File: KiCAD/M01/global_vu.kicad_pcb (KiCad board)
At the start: 2 copper layers, 100 x 49 mm, 70 parts, among them J1 Conn_01x05, J2 Conn_01x05, U1 74HC595, U2 74HC595, U3 74HC595, U4 74HC595

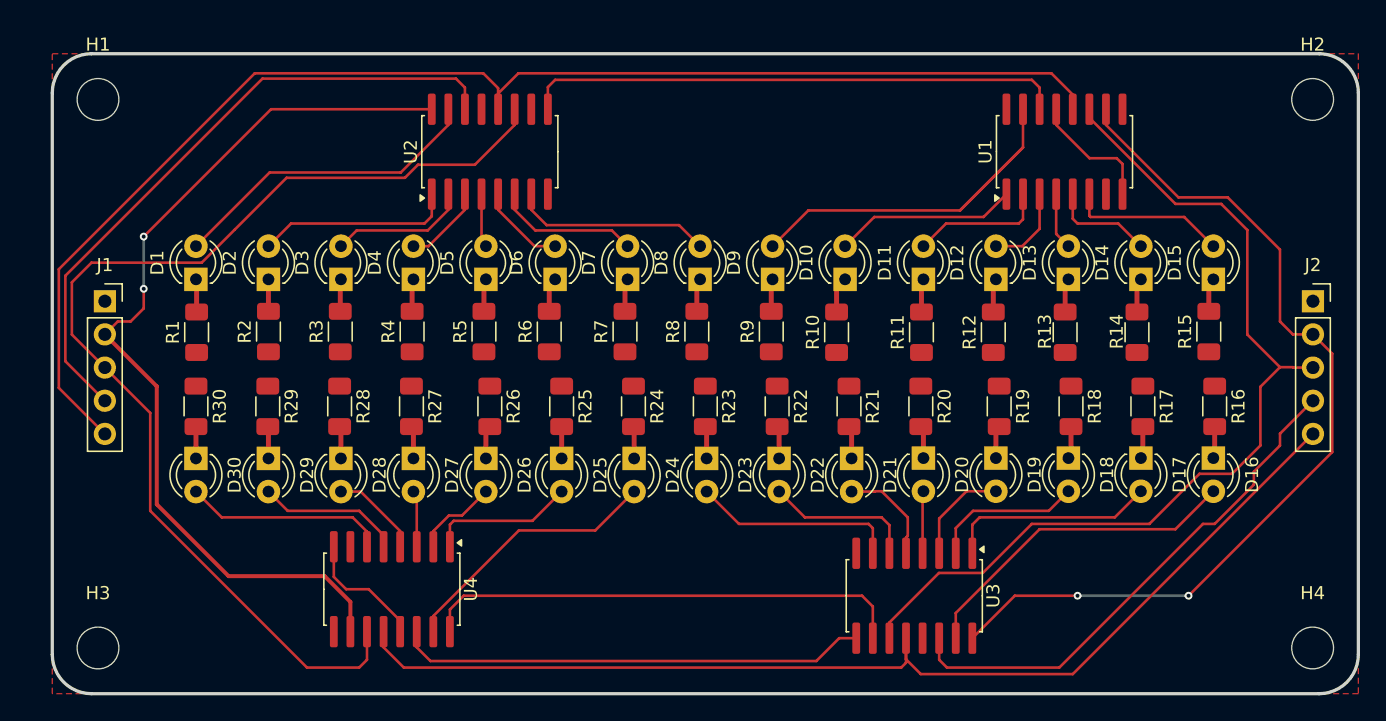
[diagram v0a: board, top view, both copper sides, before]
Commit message: chore: Update KiCAD gerber and drill files
Signed-off-by: Jose Vega <josevega234@gmail.com>
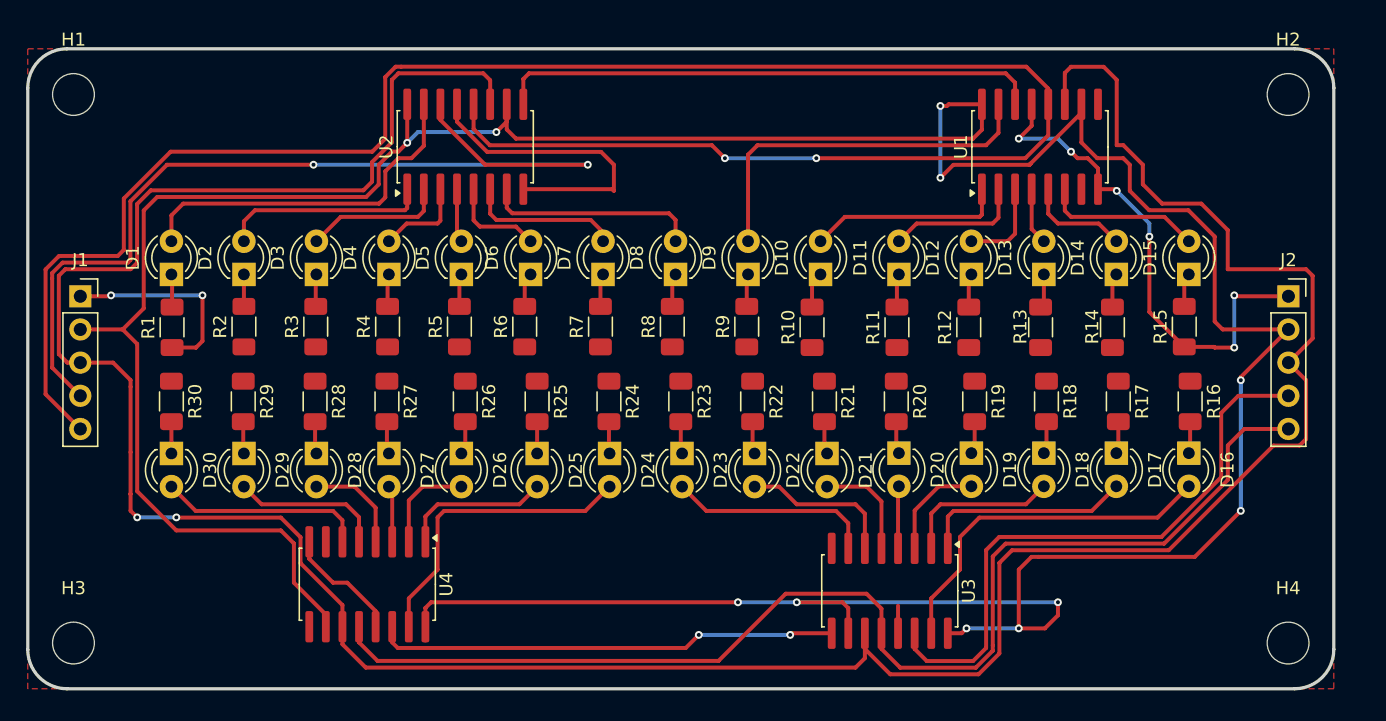
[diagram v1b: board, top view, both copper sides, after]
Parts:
- moved D21 1.92 mm to (88.8, 76.1)
- moved D22 1.92 mm to (83.3, 76.1)
- moved D24 1.92 mm to (72.2, 76.1)
- moved D25 1.92 mm to (66.6, 76.1)
- moved D26 1.92 mm to (60.8, 76.1)
- moved D28 1.92 mm to (49.7, 76.1)
- moved D30 1.92 mm to (38.6, 76.1)
- moved H4 1.92 mm to (124.1, 90.6)
- moved J2 1.92 mm to (124.1, 64.1)
- moved R10 1.92 mm to (87.7, 66.4)
- moved R11 1.92 mm to (94.2, 66.4)
- moved R12 1.92 mm to (99.7, 66.4)
- moved R13 1.92 mm to (105.2, 66.4)
- moved R14 1.92 mm to (110.7, 66.4)
- moved R15 1.92 mm to (116.2, 66.4)
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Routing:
- net +5V: track 177.5 -> 281.5 mm, vias 4 -> 11
- net /Global VU/SRCLK: track 156.3 -> 231.4 mm, vias 0 -> 2
- net GND: track 19.4 -> 89.7 mm, vias 0 -> 8
- net /Global VU/MLVU-LATCH: track 103.6 -> 153.4 mm, vias 0 -> 2
- net /Global VU/MLVU-SIG: track 49.6 -> 71.3 mm, vias 0 -> 2
- net /Global VU/MRVU-LATCH: track 84.7 -> 92.6 mm
- net /Global VU/MRVU-SIG: track 40.1 -> 45.9 mm
- net Net-(D1-A): track 24.4 -> 27.9 mm
- net Net-(D9-A): track 32.1 -> 28.7 mm
- net Net-(D24-A): track 20.5 -> 23.4 mm
- net Net-(D16-A): track 25.5 -> 27.4 mm
- net Net-(D26-A): track 6.48 -> 7.63 mm
- net Net-(D10-A): track 14.0 -> 15.1 mm
- net Net-(D8-A): track 15.3 -> 16.4 mm
- net Net-(D28-A): track 6.99 -> 7.82 mm
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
